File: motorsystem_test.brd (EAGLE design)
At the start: 100 x 80 mm, 5 parts

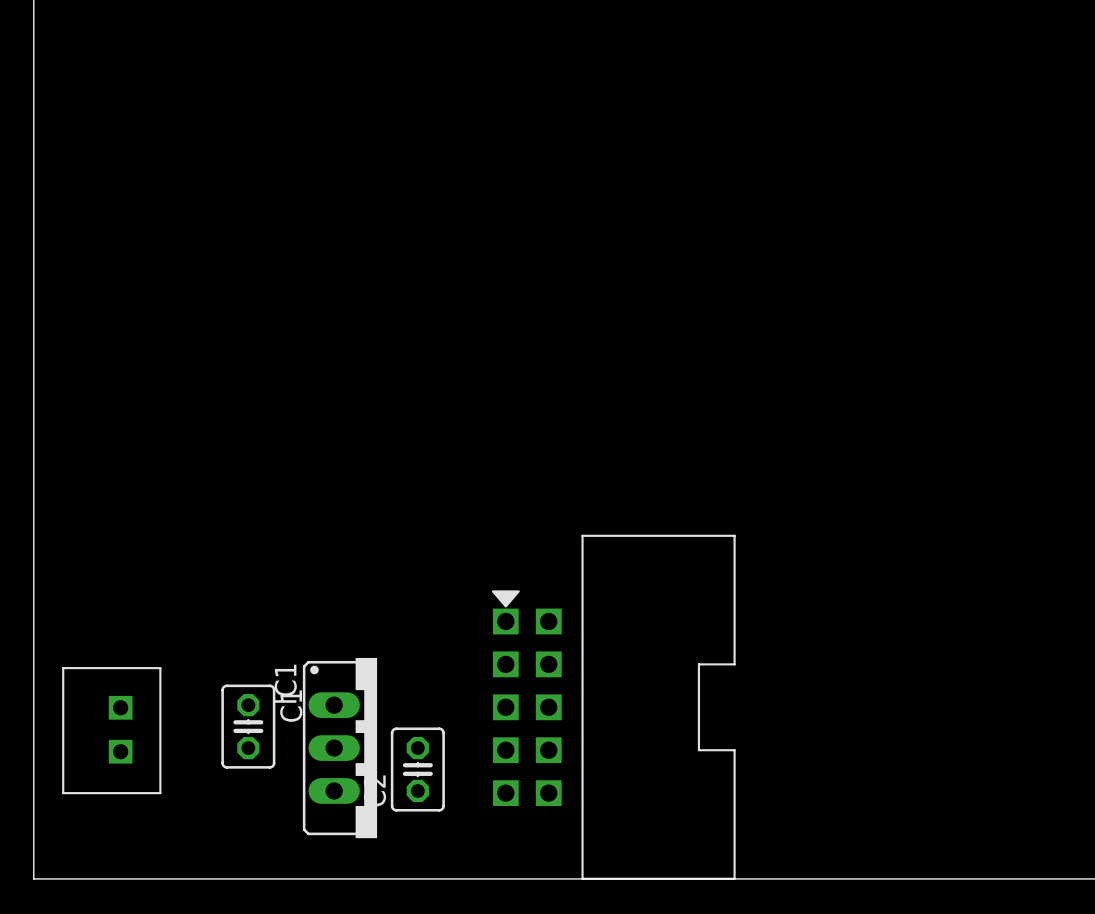
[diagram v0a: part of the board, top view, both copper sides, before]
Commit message: 図面作成
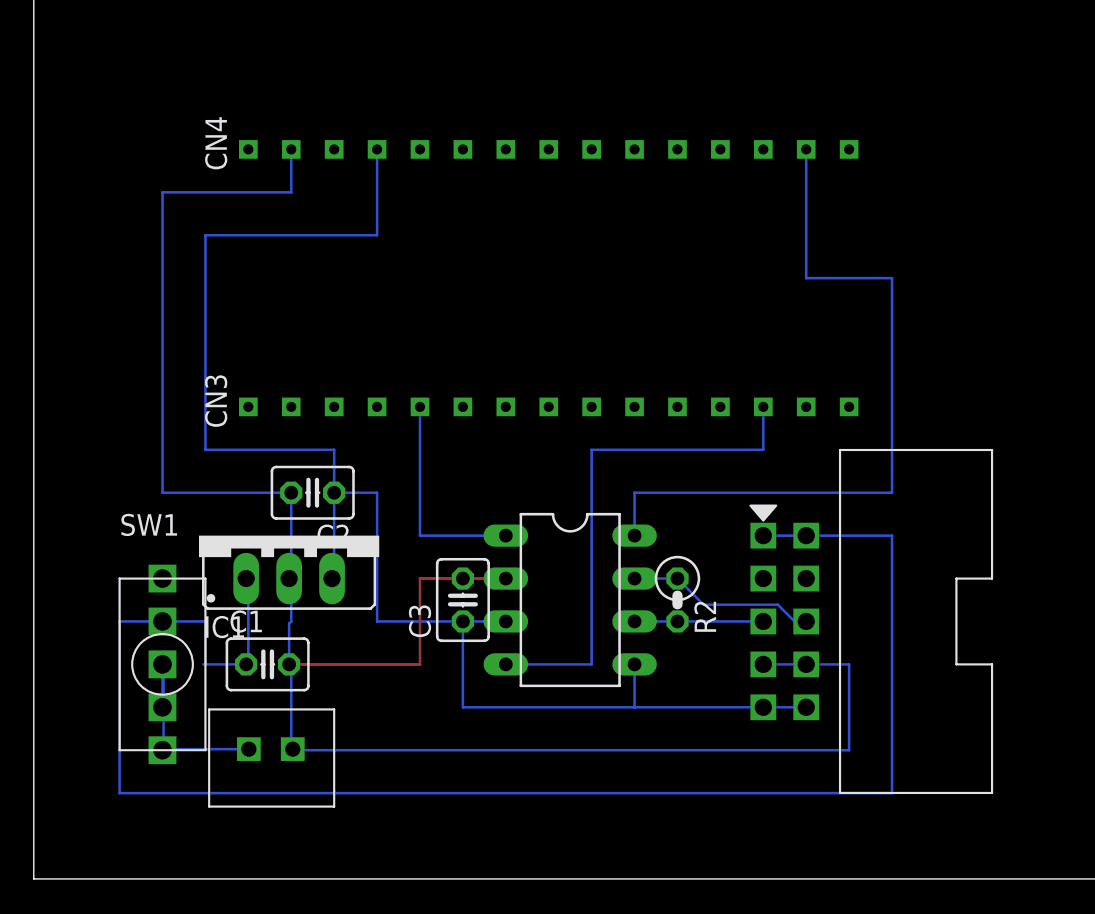
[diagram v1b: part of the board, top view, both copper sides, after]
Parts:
- added C3: 0.1u, rcl:C025-030X050
- added IC2: (no value), user_ic:DIL8
- added R2: 120, rcl:0207/2V
- added SW1: TOGURUSUIITI, user_swich:TOGURUSUIITI
- added U$3: NUCLEO-F303K8, user_ic:NUCLEO-NANO
- C1: value (none) -> 0.47u
- C2: value (none) -> 0.22u
- moved C2 17.5 mm to (16.5, 22.9), turned to 180 degrees
- moved U$2 16.1 mm to (45.7, 15.2)
- moved IC1 13.6 mm to (15.1, 20.3), turned to 0 degrees
- moved U$1 11.4 mm to (17.8, 10.0), turned to 180 degrees
- moved C1 3.86 mm to (13.8, 12.7), turned to 0 degrees
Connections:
- removed net N$3: U$2.P$5
- removed net N$4: U$2.P$6
- new net CANH: IC2.PIN6, R2.2, U$2.P$5
- new net CANL: IC2.PIN7, R2.1, U$2.P$6
- new net CAN_RX: IC2.PIN4, U$3.P$13
- new net CAN_TX: IC2.PIN1, U$3.P$5
- new net N$1: SW1.2, SW1.C, U$1.P$2
- new net N$7: IC2.PIN8, U$3.P$17
- net +12V: now also SW1.1; no longer U$1.P$2
- net +5V: now also C3.1, IC2.PIN3, IC2.PIN5, U$3.P$27
- net GND: now also C3.2, IC2.PIN2, U$3.P$29
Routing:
- net GND: track 0.00 -> 114.7 mm
- net +12V: track 0.00 -> 94.3 mm
- net +5V: track 0.00 -> 89.0 mm
- net N$7: track 0.00 -> 43.2 mm
- net CAN_RX: track 0.00 -> 30.5 mm
- net CAN_TX: track 0.00 -> 12.7 mm
- net N$1: track 0.00 -> 12.6 mm
- net CANL: track 0.00 -> 11.2 mm
- net CANH: track 0.00 -> 7.62 mm
